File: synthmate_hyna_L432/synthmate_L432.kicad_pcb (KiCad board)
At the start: 4 copper layers, 28.1 x 38.8 mm, 52 parts, among them J1 USB4105-GF-A-120, J3 Conn_01x02, J8 Conn_ST_STDC14, SW1 RotaryEncoder_Switch, SW2 PB_86_A1, SW3 PB_86_A1, SW5 PB_86_A1, U1 STM32L432KBU6, U2 TS3USB221ARSER, U3 MIC5365-3.3YC5, U4 SN74LV1T34DBVR, U5 M95M04-DRMN6TP, U6 SN74LV14APWR

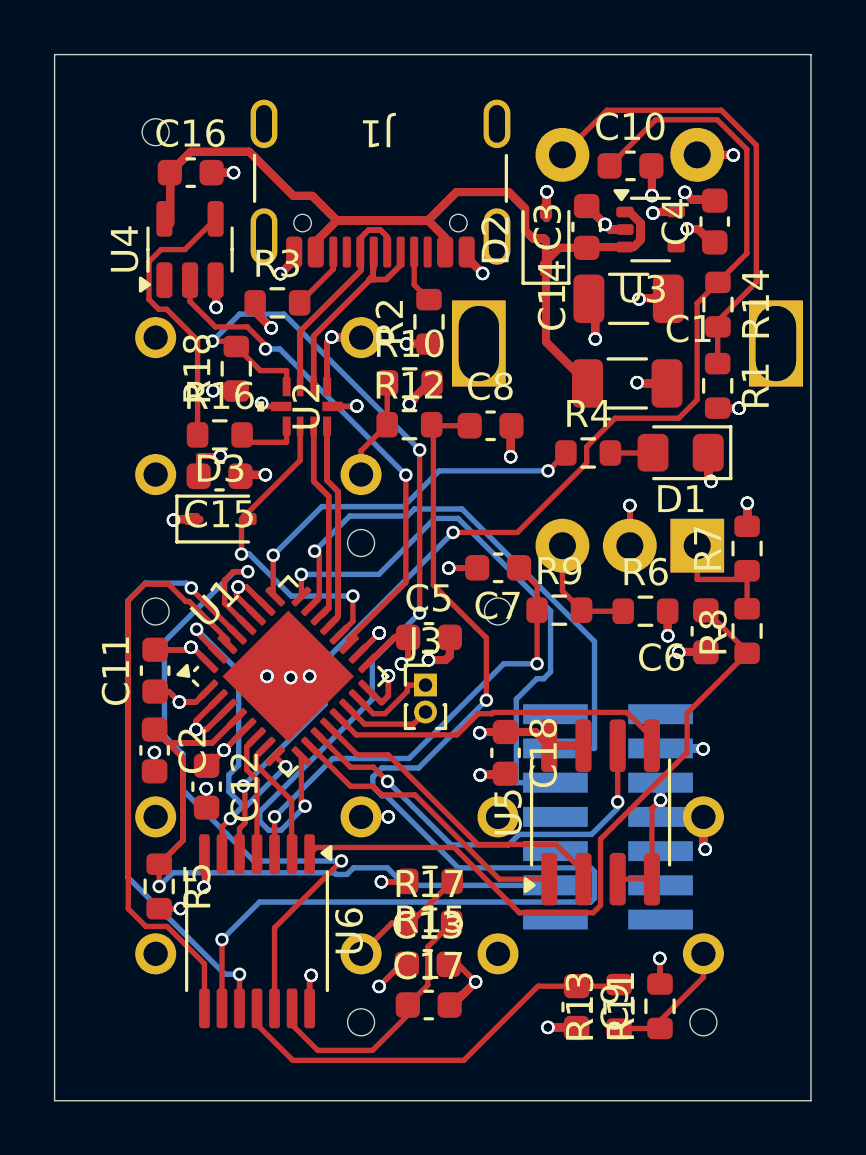
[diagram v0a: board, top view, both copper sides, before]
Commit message: 23_1
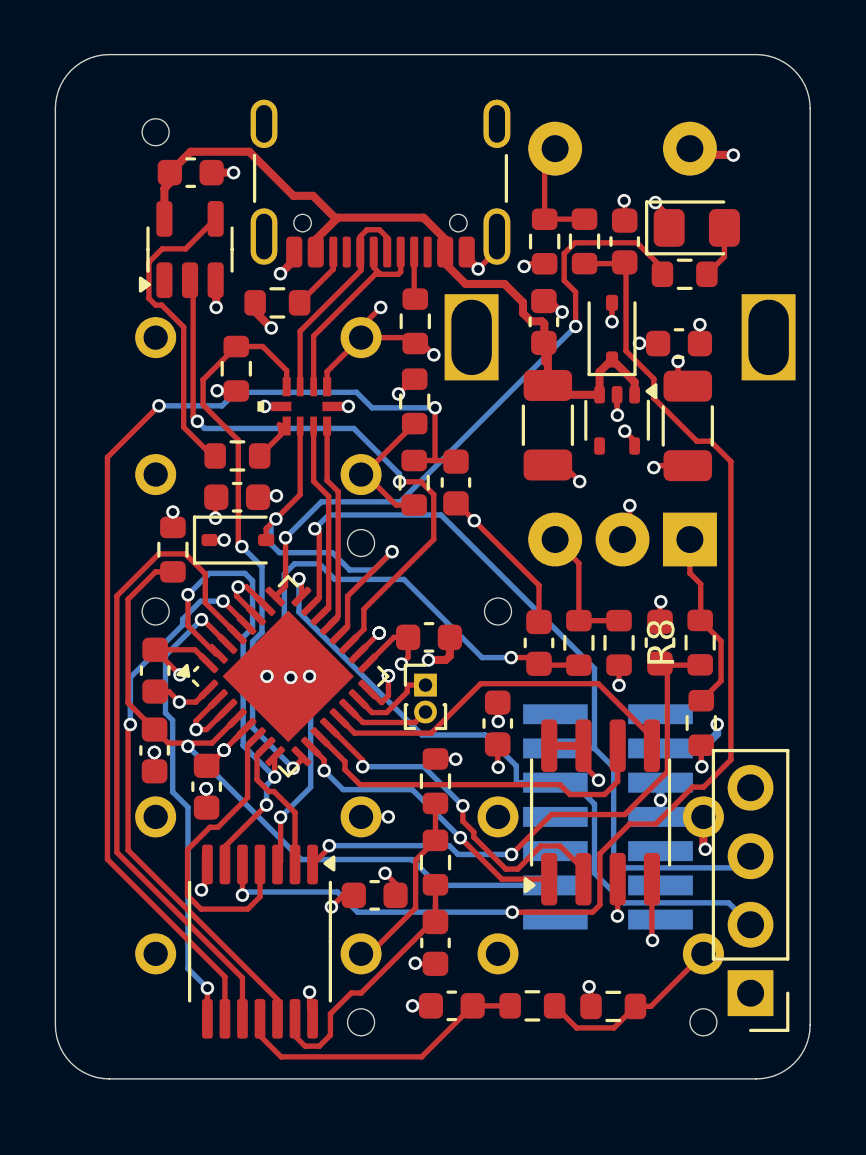
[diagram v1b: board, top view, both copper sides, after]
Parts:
- added J5: Conn_01x04, Connector_PinHeader_2.54mm:PinHeader_1x04_P2.54mm_Vertical, F.Cu at (151.6, 105.6)
- U3: value MIC5365-3.3YC5 -> MIC5365-3.3YC5-TR
- moved R5 12.5 mm to (130.2, 89.1), turned to 90 degrees
- moved D1 8.36 mm to (149.6, 77.2), turned to 0 degrees
- moved R1 8.36 mm to (144.0, 77.7)
- moved R4 7.53 mm to (149.2, 78.9)
- moved U3 7.19 mm to (146.7, 84.3), turned to -90 degrees
- moved R7 6.69 mm to (149.8, 95.6), turned to -90 degrees
- moved R14 5.48 mm to (145.4, 77.7), turned to 90 degrees
- moved C14 5.20 mm to (149.3, 84.6), turned to -90 degrees
- moved C4 4.72 mm to (149.0, 81.5), turned to 180 degrees
- moved C9 4.64 mm to (140.5, 106.1), turned to 180 degrees
- moved D2 4.18 mm to (146.5, 81.0)
- moved C3 3.87 mm to (143.9, 80.7)
- moved R15 3.72 mm to (139.9, 97.7), turned to 90 degrees
- moved C1 3.33 mm to (144.1, 84.5), turned to -90 degrees
- moved C13 3.23 mm to (137.7, 102.0)
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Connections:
- U5 pad 3: GND -> 3V3
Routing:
- net GND: track 109.6 -> 59.6 mm, vias 80 -> 45
- net 5V: track 65.9 -> 30.2 mm
- net 3V3: track 60.0 -> 29.4 mm, vias 45 -> 24
- net usb_switch: track 34.3 -> 21.2 mm, vias 4 -> 2
- net Net-(R1-Pad1): track 17.1 -> 4.26 mm
- net LED: track 14.0 -> 23.7 mm
- net SWDIO: track 20.7 -> 30.2 mm
- net NRST: track 35.0 -> 26.9 mm
- net /usb_N: track 15.8 -> 7.77 mm
- net /usb_P: track 16.3 -> 8.40 mm
- net /usb_mcu_N: track 15.4 -> 7.90 mm
- net Net-(C7-Pad1): track 17.3 -> 24.7 mm
- net /usb_mcu_P: track 15.0 -> 7.60 mm
- net enc_B: track 4.64 -> 11.4 mm
- net Net-(C8-Pad1): track 45.7 -> 39.6 mm
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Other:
- board size 28.1 x 38.8 mm -> 28 x 38 mm
- board text added: "3V3 SWDIO SWCLK GND"
